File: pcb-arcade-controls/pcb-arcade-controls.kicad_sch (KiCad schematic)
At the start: 20 parts, among them J1 USB_C, SW1 SW_Push, U1 STM32F072CBT6, U3 XC6206, U4 USBLC6-2SC6

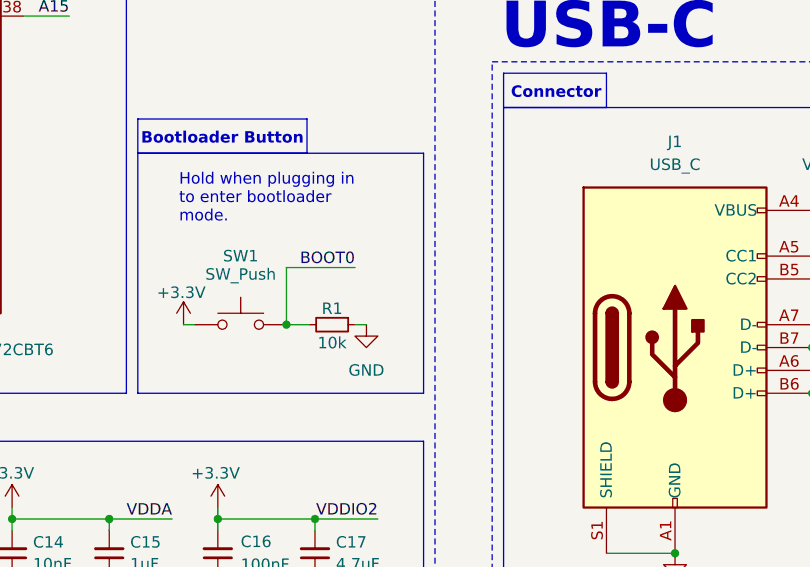
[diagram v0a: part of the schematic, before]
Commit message: start aan pcb
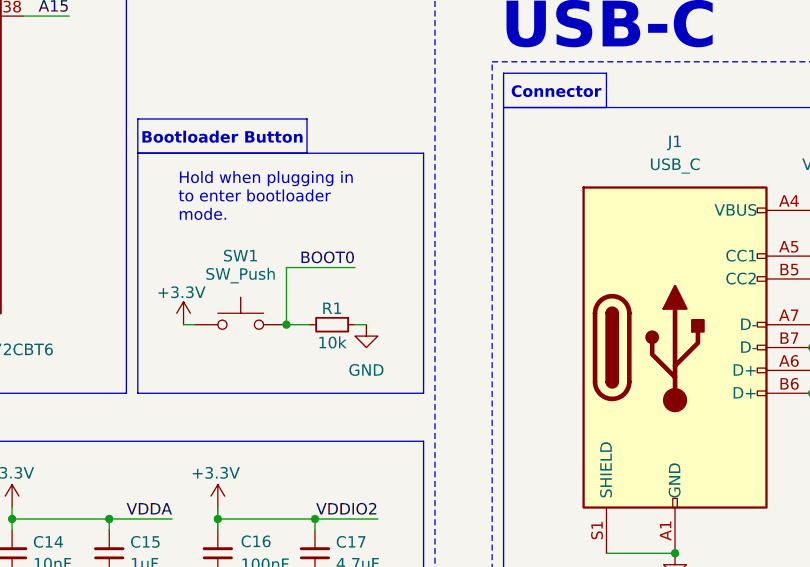
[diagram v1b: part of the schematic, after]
